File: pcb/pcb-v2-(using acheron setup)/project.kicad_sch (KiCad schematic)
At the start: 174 parts, among them J1 Conn_01x22_Female, J2 Conn_01x22_Male, J3 Conn_01x03_Male, J4 helios, SW1 CherryMX, SW10 CherryMX, SW11 CherryMX, SW12 CherryMX, SW13 CherryMX, SW14 CherryMX, SW15 CherryMX, SW16 CherryMX, SW17 CherryMX, SW18 CherryMX, SW19 CherryMX, SW2 CherryMX, SW20 CherryMX, SW21 CherryMX, SW22 CherryMX, SW23 CherryMX, SW24 CherryMX, SW25 CherryMX, SW26 CherryMX, SW27 CherryMX, SW28 CherryMX, SW29 CherryMX, SW3 CherryMX, SW30 CherryMX, SW31 CherryMX, SW32 CherryMX, SW33 CherryMX, SW34 CherryMX, SW35 CherryMX, SW36 CherryMX, SW37 CherryMX, SW38 CherryMX, SW39 CherryMX, SW4 CherryMX, SW40 CherryMX, SW41 CherryMX, SW42 CherryMX, SW43 CherryMX, SW44 CherryMX, SW45 CherryMX, SW46 CherryMX, SW47 CherryMX, SW48 CherryMX, SW49 CherryMX, SW5 CherryMX, SW50 CherryMX, SW51 CherryMX, SW52 CherryMX, SW53 CherryMX, SW54 CherryMX, SW55 CherryMX, SW56 CherryMX, SW57 CherryMX, SW58 CherryMX, SW59 CherryMX, SW6 CherryMX, SW60 CherryMX, SW61 CherryMX, SW62 CherryMX, SW63 CherryMX, SW64 CherryMX, SW65 CherryMX, SW66 CherryMX, SW67 CherryMX, SW68 CherryMX, SW69 CherryMX, SW7 CherryMX, SW70 CherryMX, SW71 CherryMX, SW72 CherryMX, SW73 CherryMX, SW74 CherryMX, SW75 CherryMX, SW76 CherryMX, SW77 CherryMX, SW78 CherryMX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

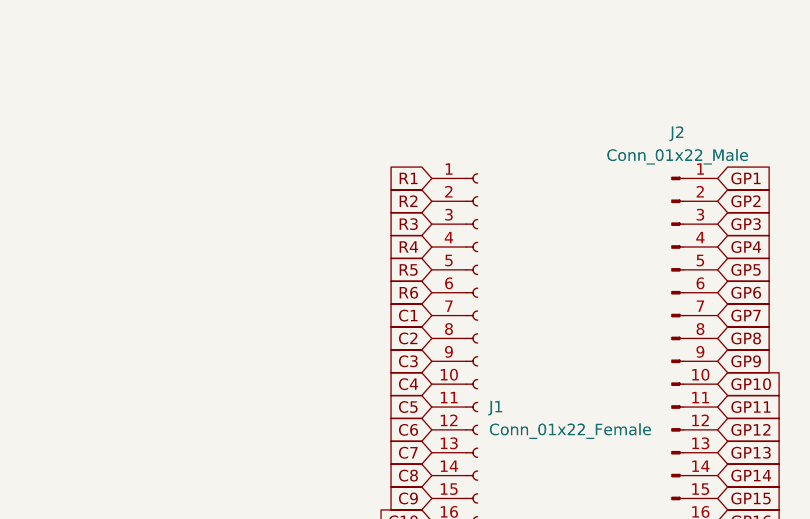
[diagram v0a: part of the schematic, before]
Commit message: draft routing complete now refining ig
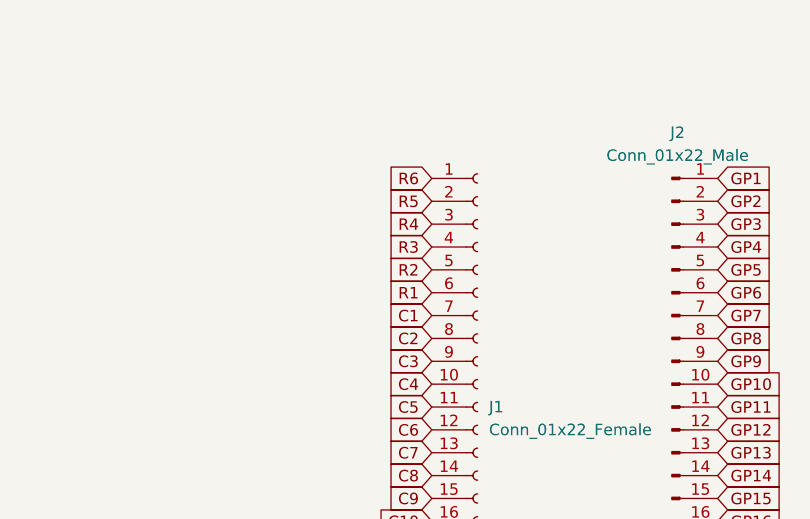
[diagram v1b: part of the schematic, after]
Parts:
- SW36: footprint CherryMX:CherryMX_6.00u -> CherryMX_StabWireBottom:CherryMX_6.00u_StabWireBottom
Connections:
- net R1: now also J1.6 (Pin_6); no longer J1.1 (Pin_1)
- net R2: now also J1.5 (Pin_5); no longer J1.2 (Pin_2)
- net R3: now also J1.4 (Pin_4); no longer J1.3 (Pin_3)
- net R4: now also J1.3 (Pin_3); no longer J1.4 (Pin_4)
- net R5: now also J1.2 (Pin_2); no longer J1.5 (Pin_5)
- net R6: now also J1.1 (Pin_1); no longer J1.6 (Pin_6)
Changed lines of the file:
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@@
     )
   )
-  (global_label "R5" (shape input) (at 295.91 69.85 180) (fields_autoplaced)
+  (global_label "R5" (shape input) (at 295.91 62.23 180) (fields_autoplaced)
     (effects (font (size 1.27 1.27)) (justify right))
-    (property "Intersheet References" "${INTERSHEET_REFS}" (id 0) (at 291.0174 69.7706 0)
+    (property "Intersheet References" "${INTERSHEET_REFS}" (id 0) (at 291.0174 62.3094 0)
       (effects (font (size 1.27 1.27)) (justify right) hide)
     )
@@
     )
   )
-  (global_label "R2" (shape input) (at 295.91 62.23 180) (fields_autoplaced)
+  (global_label "R2" (shape input) (at 295.91 69.85 180) (fields_autoplaced)
     (effects (font (size 1.27 1.27)) (justify right))
-    (property "Intersheet References" "${INTERSHEET_REFS}" (id 0) (at 291.0174 62.1506 0)
+    (property "Intersheet References" "${INTERSHEET_REFS}" (id 0) (at 291.0174 69.9294 0)
       (effects (font (size 1.27 1.27)) (justify right) hide)
     )
@@
     )
   )
-  (global_label "R1" (shape input) (at 295.91 59.69 180) (fields_autoplaced)
+  (global_label "R1" (shape input) (at 295.91 72.39 180) (fields_autoplaced)
     (effects (font (size 1.27 1.27)) (justify right))
-    (property "Intersheet References" "${INTERSHEET_REFS}" (id 0) (at 291.0174 59.6106 0)
+    (property "Intersheet References" "${INTERSHEET_REFS}" (id 0) (at 291.0174 72.4694 0)
       (effects (font (size 1.27 1.27)) (justify right) hide)
     )
@@
     )
   )
-  (global_label "R3" (shape input) (at 295.91 64.77 180) (fields_autoplaced)
+  (global_label "R3" (shape input) (at 295.91 67.31 180) (fields_autoplaced)
     (effects (font (size 1.27 1.27)) (justify right))
-    (property "Intersheet References" "${INTERSHEET_REFS}" (id 0) (at 291.0174 64.6906 0)
+    (property "Intersheet References" "${INTERSHEET_REFS}" (id 0) (at 291.0174 67.3894 0)
       (effects (font (size 1.27 1.27)) (justify right) hide)
     )
@@
     )
   )
-  (global_label "R6" (shape input) (at 295.91 72.39 180) (fields_autoplaced)
+  (global_label "R6" (shape input) (at 295.91 59.69 180) (fields_autoplaced)
     (effects (font (size 1.27 1.27)) (justify right))
-    (property "Intersheet References" "${INTERSHEET_REFS}" (id 0) (at 291.0174 72.3106 0)
+    (property "Intersheet References" "${INTERSHEET_REFS}" (id 0) (at 291.0174 59.7694 0)
       (effects (font (size 1.27 1.27)) (justify right) hide)
     )
@@
     )
   )
-  (global_label "R4" (shape input) (at 295.91 67.31 180) (fields_autoplaced)
+  (global_label "R4" (shape input) (at 295.91 64.77 180) (fields_autoplaced)
     (effects (font (size 1.27 1.27)) (justify right))
-    (property "Intersheet References" "${INTERSHEET_REFS}" (id 0) (at 291.0174 67.2306 0)
+    (property "Intersheet References" "${INTERSHEET_REFS}" (id 0) (at 291.0174 64.8494 0)
       (effects (font (size 1.27 1.27)) (justify right) hide)
     )
@@
     (property "Reference" "SW36" (id 0) (at 116.84 119.38 0))
     (property "Value" "CherryMX" (id 1) (at 116.84 121.92 0))
-    (property "Footprint" "CherryMX:CherryMX_6.00u" (id 2) (at 116.84 126.365 0)
+    (property "Footprint" "CherryMX_StabWireBottom:CherryMX_6.00u_StabWireBottom" (id 2) (at 116.84 126.365 0)
       (effects (font (size 1.27 1.27)) hide)
     )
@@
     )
     (path "/5b501776-44a9-42cb-867a-253c7bce0f28"
-      (reference "SW36") (unit 1) (value "CherryMX") (footprint "CherryMX:CherryMX_6.00u")
+      (reference "SW36") (unit 1) (value "CherryMX") (footprint "CherryMX_StabWireBottom:CherryMX_6.00u_StabWireBottom")
     )
     (path "/76019206-3da3-478e-85c9-55c50424b5ff"
